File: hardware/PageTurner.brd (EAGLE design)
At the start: 100 x 80 mm, 12 parts

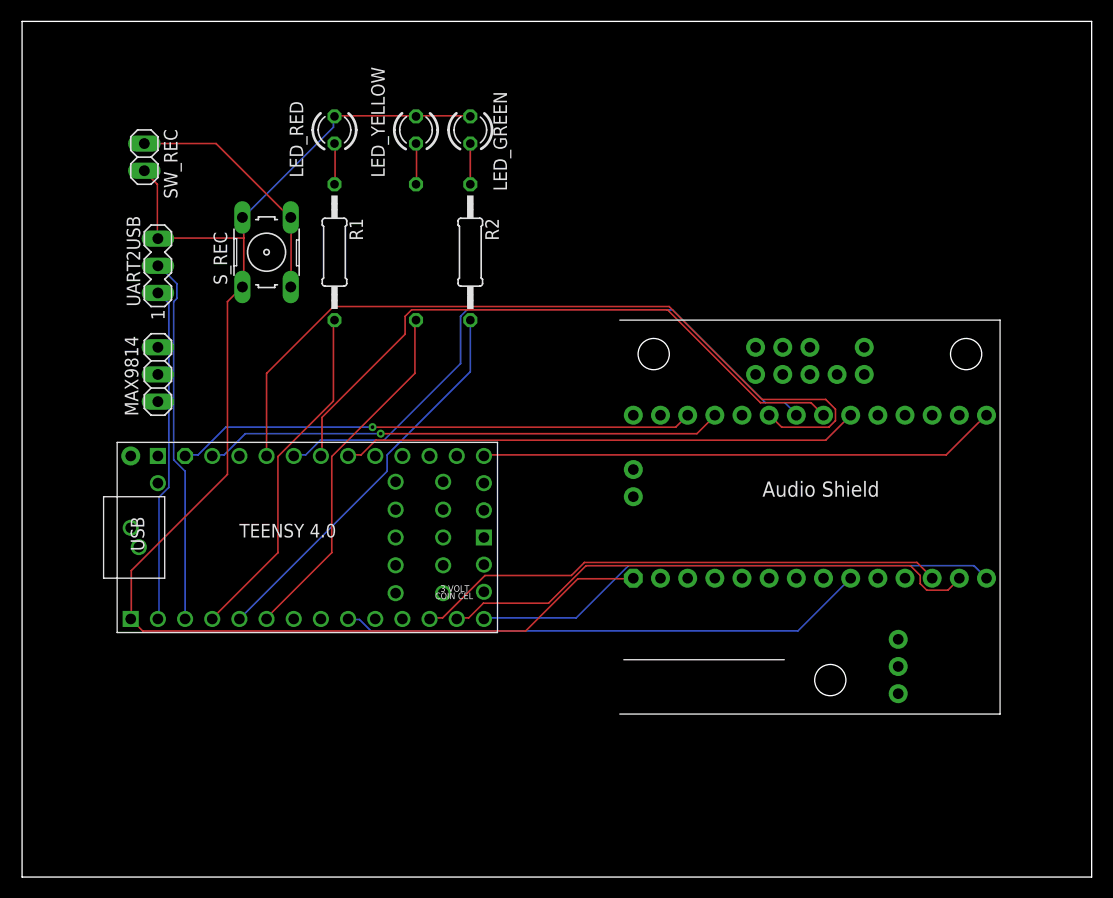
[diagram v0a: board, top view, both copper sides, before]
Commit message: preparations for futrue improvements
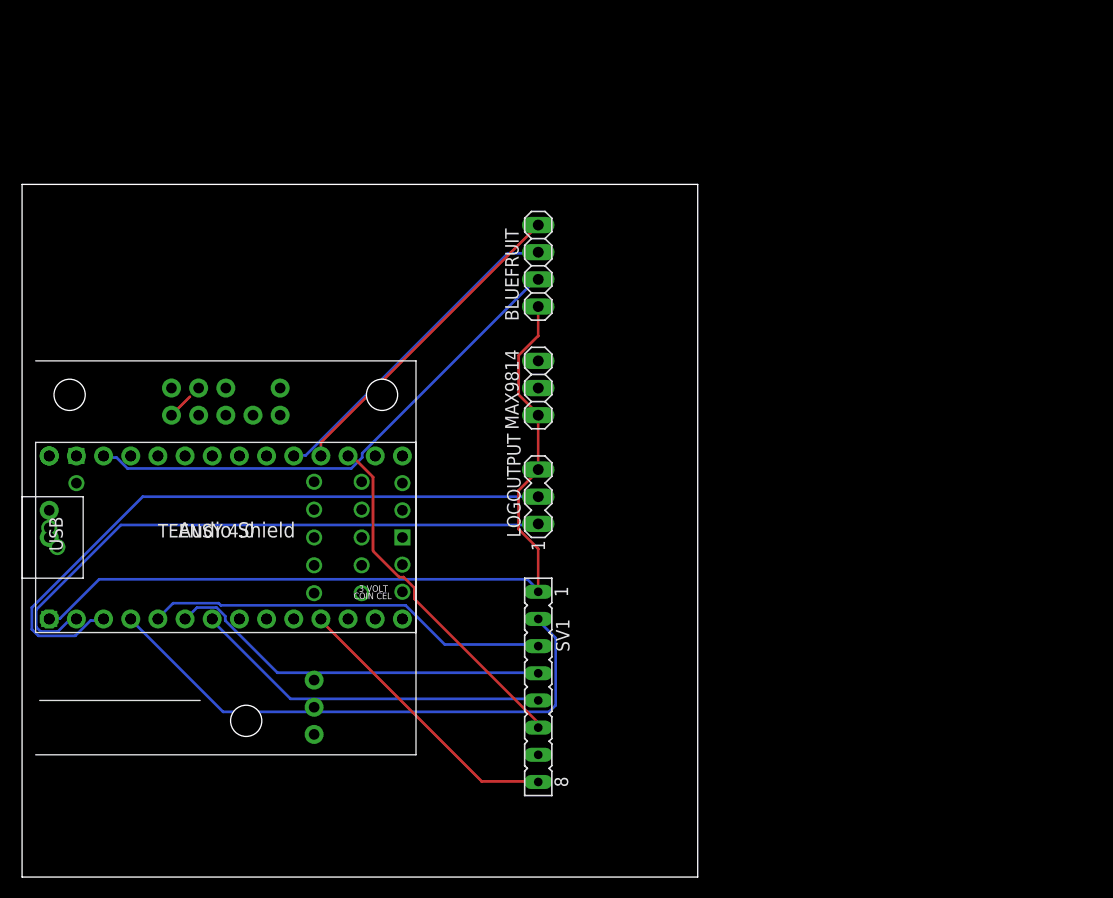
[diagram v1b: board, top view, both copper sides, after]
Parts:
- removed LED_GREEN, LED_RED, LED_YELLOW: (no value), led:LED3MM
- removed R1, R2, R3: 470, rcl:0207/12
- removed SW_REC: (no value), pinhead:1X02
- removed S_REC: (no value), switch-omron:B3F-10XX
- removed UART2USB: (no value), con-lstb:MA03-1
- added BLUEFRUIT: (no value), pinhead:1X04
- added LOGOUTPUT: (no value), con-lstb:MA03-1
- added SV1: (no value), con-lsta:FE08
- moved U$2 54.7 mm to (19.1, 29.2)
- moved MAX9814 35.6 mm to (48.3, 45.7)
- moved U$1 7.62 mm to (19.1, 31.8)
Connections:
- removed net N$13: U$1.20-A6/TX5/LRCLK1, U$2.20
- removed net N$14: U$1.19-A5/SCL0, U$2.19
- removed net N$15: U$1.7-RX2/OUT1A, U$2.7
- removed net N$16: U$1.18-A4/SDA0, U$2.18
- removed net N$17: U$1.10-CS/MQSR, U$2.10
- removed net N$19: U$1.11-MOSI/CTX1, U$2.11
- removed net N$20: U$1.12-MIO/MQSL, U$2.12
- removed net N$21: U$1.13-SCK/CRX1/LED, U$2.13
- removed net N$4: LED_YELLOW.A, R3.1
- removed net N$7: LED_GREEN.K, LED_RED.K, LED_YELLOW.K, SW_REC.2, S_REC.1, S_REC.2, U$1.GND1, U$2.G, U$2.GND, UART2USB.3
- new net 3V: MAX9814.2, U$2.3V
- new net BLE_RX: BLUEFRUIT.3, U$1.17-A3/TX4/SDA1
- new net BLE_TX: BLUEFRUIT.4, U$1.16-A2/RX4/SCL1
- net 3.3V: now also BLUEFRUIT.2; no longer MAX9814.2, U$2.3V
- net GND: now also BLUEFRUIT.1, LOGOUTPUT.3, SV1.1, U$1.GND1; no longer U$2.INGND1
- net N$1: now also SV1.2; no longer R1.2
- net N$10: now also LOGOUTPUT.2; no longer UART2USB.2
- net N$11: now also SV1.5, U$1.5-IN2; no longer U$1.23-A9/CRX1/CCLK1, U$2.23
- net N$12: now also SV1.6, U$1.15-A1/RX3/S-PDIF_IN; no longer U$1.21-A7/RX5/BCLK1, U$2.21
- net N$2: now also SV1.7; no longer R2.2, U$1.3-LRCLK2
- net N$3: now also SV1.8, U$1.9-OUT1C; no longer R3.2, U$1.4-BCLK2
- net N$5: now also U$1.14-A0/TX3/S-PFI_OUT; no longer LED_GREEN.A, R2.1
- net N$6: now also SV1.3, U$1.3-LRCLK2; no longer LED_RED.A, R1.1
- net N$8: now also LOGOUTPUT.1; no longer UART2USB.1
- net N$9: now also SV1.4, U$1.4-BCLK2; no longer SW_REC.1, S_REC.3, S_REC.4, U$1.5-IN2
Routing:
- net N$7: track 132.4 -> 0.00 mm
- net GND: track 0.00 -> 77.6 mm
- net N$14: track 59.8 -> 0.00 mm
- net N$13: track 59.4 -> 0.00 mm
- net N$19: track 51.0 -> 0.00 mm
- net N$17: track 49.9 -> 0.00 mm
- net N$20: track 49.5 -> 0.00 mm
- net N$15: track 49.5 -> 0.00 mm
- net N$16: track 48.6 -> 0.00 mm
- net N$21: track 48.6 -> 0.00 mm
- net N$12: track 75.4 -> 33.2 mm
- net N$2: track 36.9 -> 0.00 mm
- net N$6: track 3.91 -> 38.0 mm
- net BLE_RX: track 0.00 -> 30.8 mm
- net BLE_TX: track 0.00 -> 30.0 mm
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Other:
- board size 100 x 80 mm -> 63.2 x 64.8 mm
